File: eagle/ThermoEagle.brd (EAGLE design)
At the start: 100 x 80 mm, 35 parts, among them IC1 MAX232, IC2 4511N, Q1 20MHz, T1 2N2219, T2 2N2219, U1 LM324

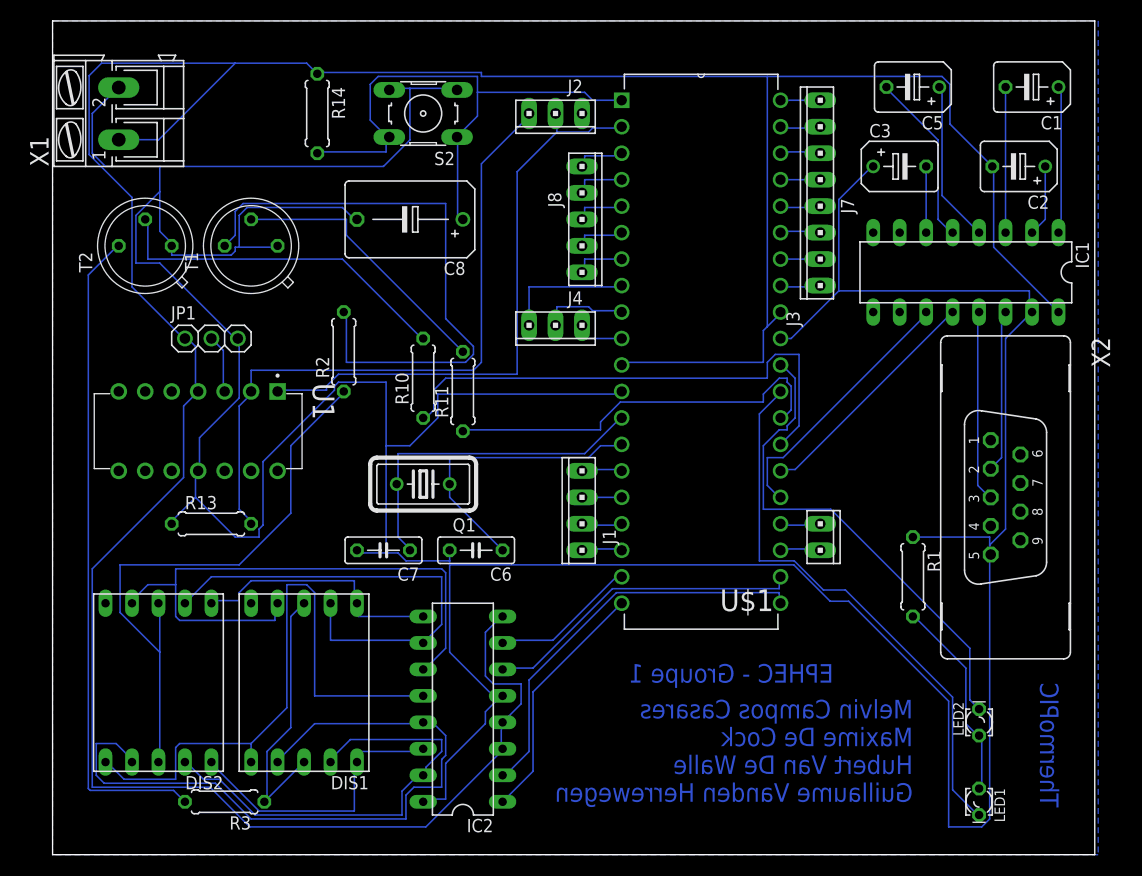
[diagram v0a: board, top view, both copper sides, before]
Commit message: Update Board - validation #2 by EuroCircuit
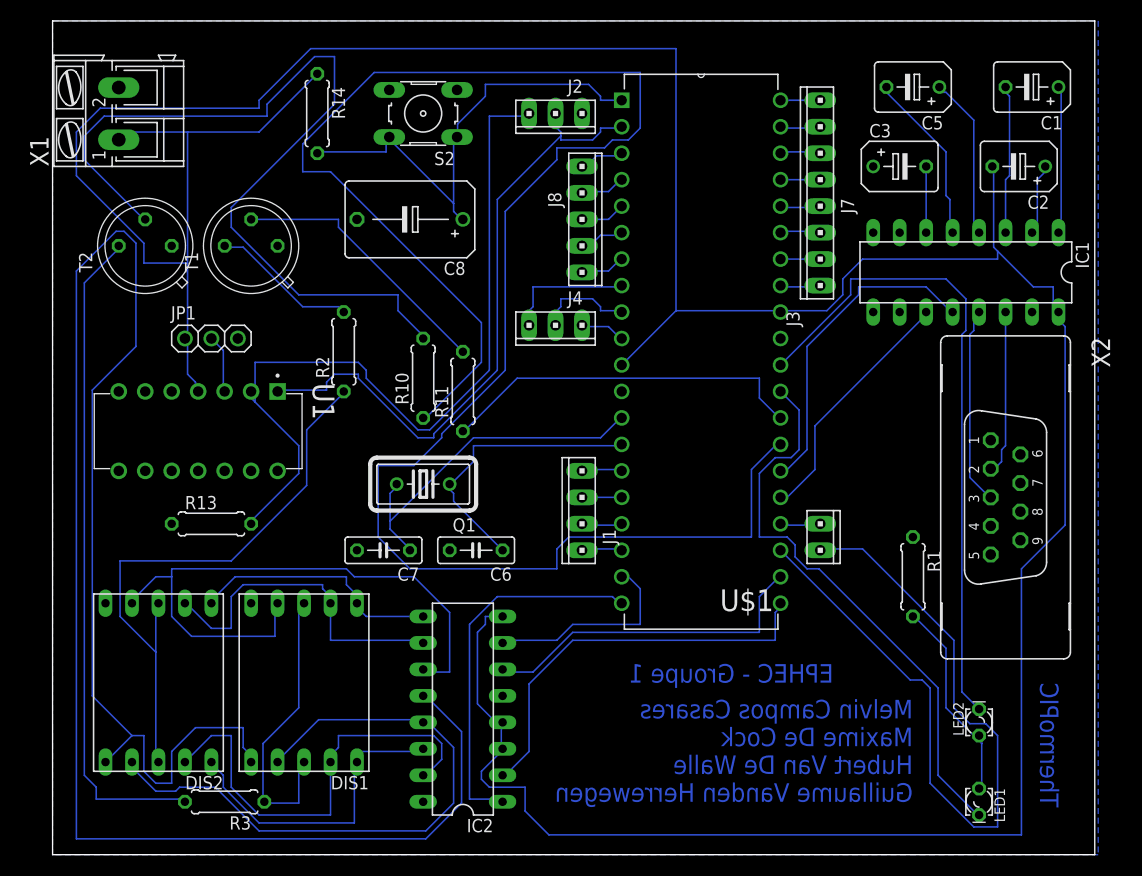
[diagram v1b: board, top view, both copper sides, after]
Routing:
- net GND: track 410.0 -> 0.00 mm
- net N$38: track 50.0 -> 183.2 mm
- net N$27: track 59.6 -> 188.9 mm
- net N$70: track 3.89 -> 74.2 mm
- net N$4: track 33.6 -> 82.8 mm
- net N$9: track 57.3 -> 14.3 mm
- net VCC: track 306.3 -> 341.2 mm
- net N$37: track 47.7 -> 63.1 mm
- net N$25: track 45.4 -> 32.4 mm
- net N$31: track 63.9 -> 76.7 mm
- net N$6: track 23.8 -> 36.2 mm
- net RX: track 22.8 -> 31.3 mm
- net N$72: track 53.7 -> 45.7 mm
- net N$28: track 68.2 -> 60.6 mm
- net N$1: track 14.1 -> 19.6 mm
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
